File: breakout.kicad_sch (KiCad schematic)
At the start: 30 parts, among them J1 Conn_02x05_Odd_Even, J10 SATA_Power_15P_Male, J2 USB_C_Receptacle_USB2.0_16P, J7 SATA_Power_15P_Male, J8 SATA_Power_15P_Male, J9 SATA_Power_15P_Male, SW1 SW_DPST_x2, U1 TPS568230, U2 CYPD3174-24LQXQ

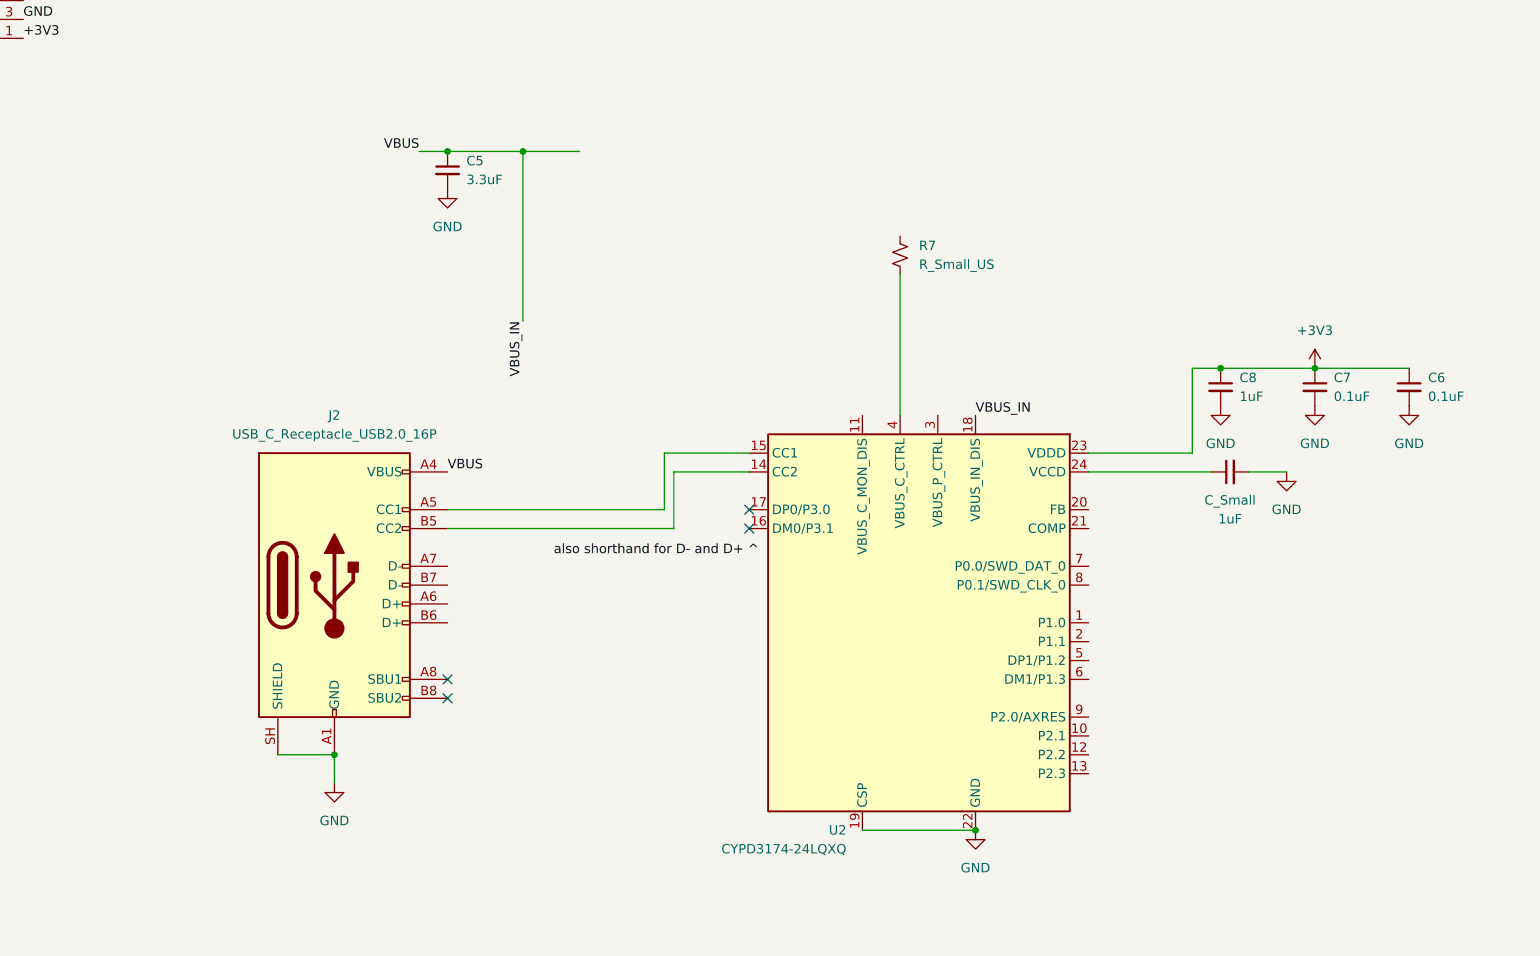
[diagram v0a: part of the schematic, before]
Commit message: feat :implement cypd3174??
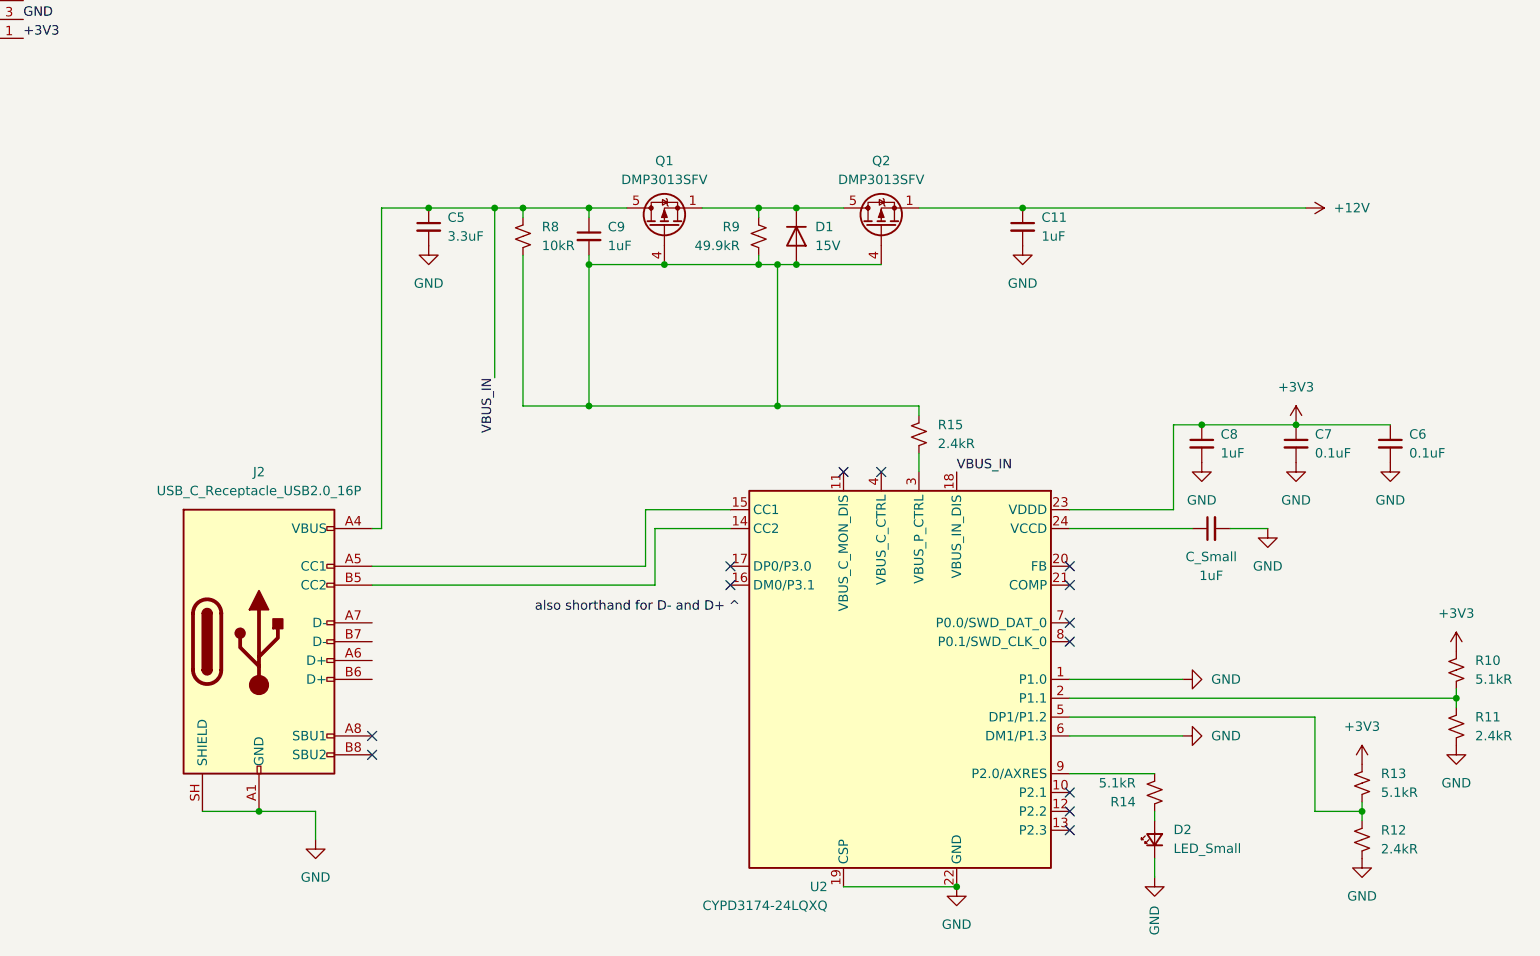
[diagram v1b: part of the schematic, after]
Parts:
- removed R7: R_Small_US, symbol Device:R_Small_US
- added C11, C9: 1uF, symbol Device:C_Small
- added D1: 15V, Diode_THT:D_DO-41_SOD81_P10.16mm_Horizontal, symbol Diode:1N4003
- added D2: LED_Small, symbol Device:LED_Small
- added Q1, Q2: DMP3013SFV, Package_SON:Diodes_PowerDI3333-8, symbol Transistor_FET:DMP3013SFV
- added R10, R13, R14: 5.1kR, symbol Device:R_Small_US
- added R11, R12, R15: 2.4kR, symbol Device:R_Small_US
- added R8: 10kR, symbol Device:R_Small_US
- added R9: 49.9kR, symbol Device:R_Small_US
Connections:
- net +12V: now also C11.1, Q2.1 (S), Q2.2 (S), Q2.3 (S)
- net +3V3: now also R10.1, R13.1
- net GND: now also U2.1 (P1.0), U2.6 (DM1/P1.3), C11.2, D2.1 (K), R11.2, R12.2
- net at U2.2 (P1.1): now also R10.2, R11.1
- net at U2.3 (VBUS_P_CTRL): now also R15.2
- net at U2.5 (DP1/P1.2): now also R12.1, R13.2
- net at U2.9 (P2.0/AXRES): now also R14.2
- net VBUS renamed VBUS_IN
- net VBUS_IN: now also C9.1, Q1.5 (D), R8.1
- new net: D2.2 (A), R14.1
- new net: C9.2, D1.2 (A), Q1.4 (G), Q2.4 (G), R15.1, R8.2, R9.2
- new net: D1.1 (K), Q1.1 (S), Q1.2 (S), Q1.3 (S), Q2.5 (D), R9.1
- no-connect marks 4 -> 13
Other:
- moved on the sheet: 1uF, C5, C6, C7, C8, J2, U2
